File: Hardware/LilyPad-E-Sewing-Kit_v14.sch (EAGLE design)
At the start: 42 parts

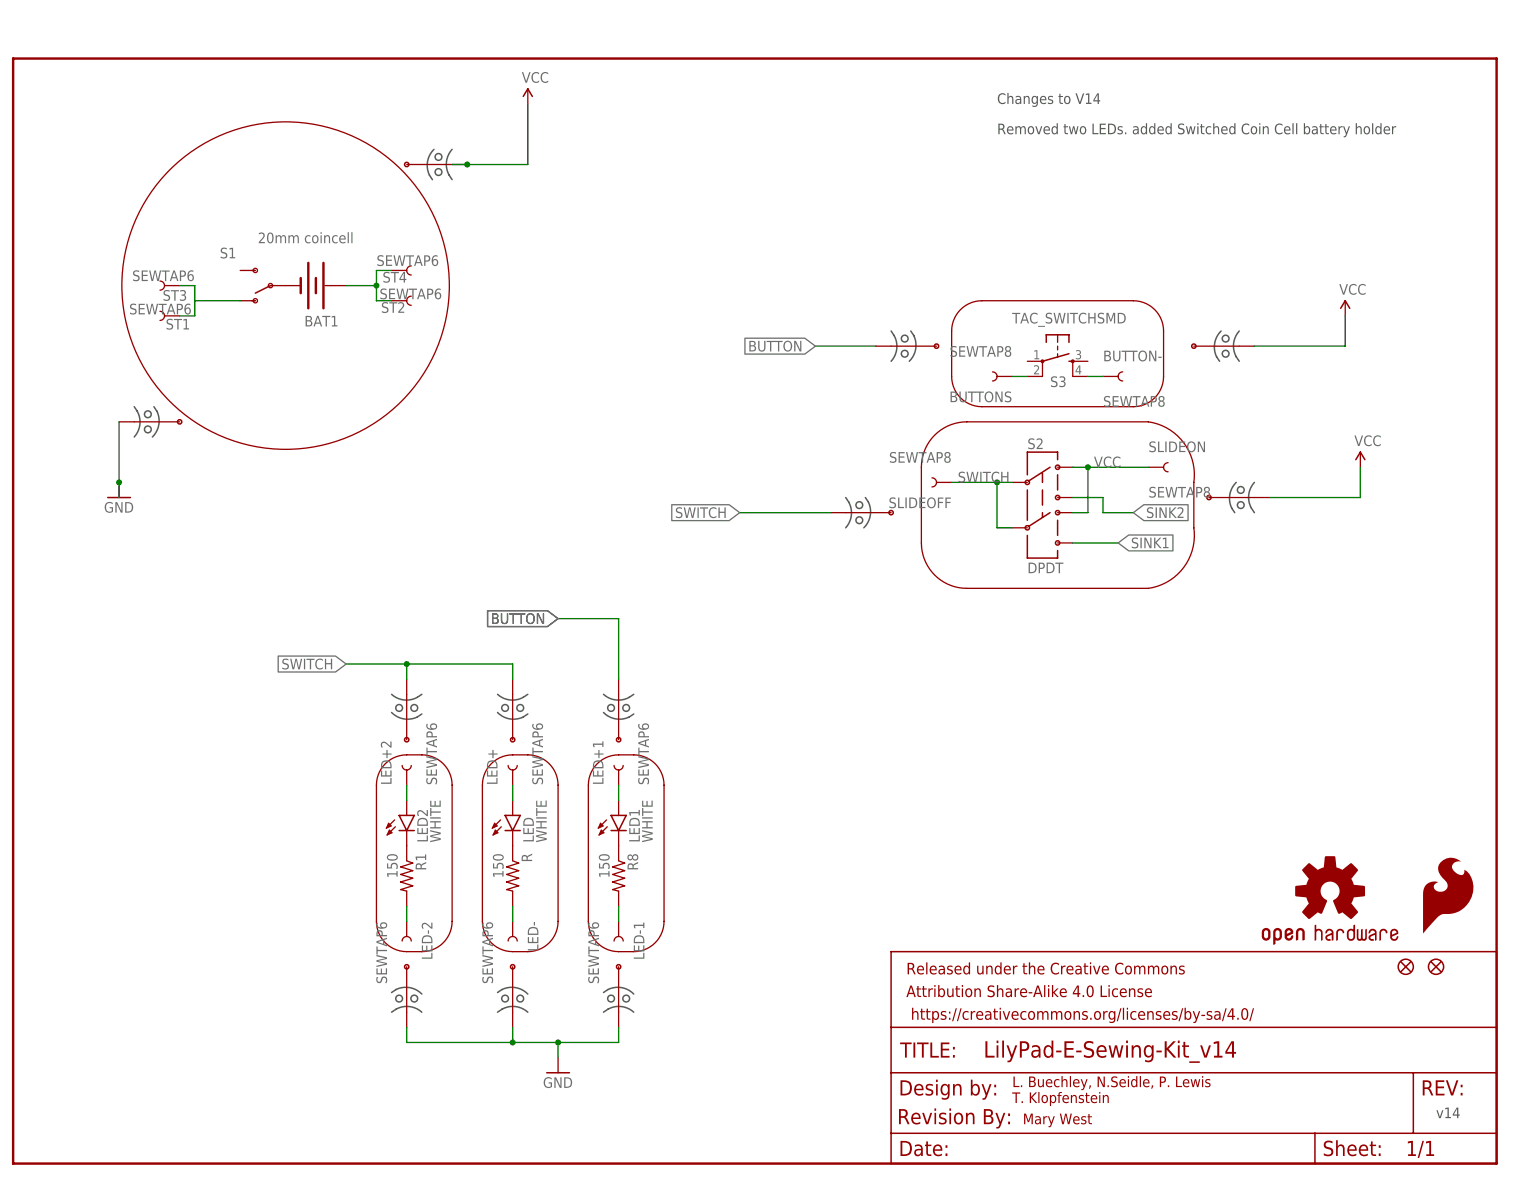
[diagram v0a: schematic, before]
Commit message: Updated Brd and Sch files (in Sync)
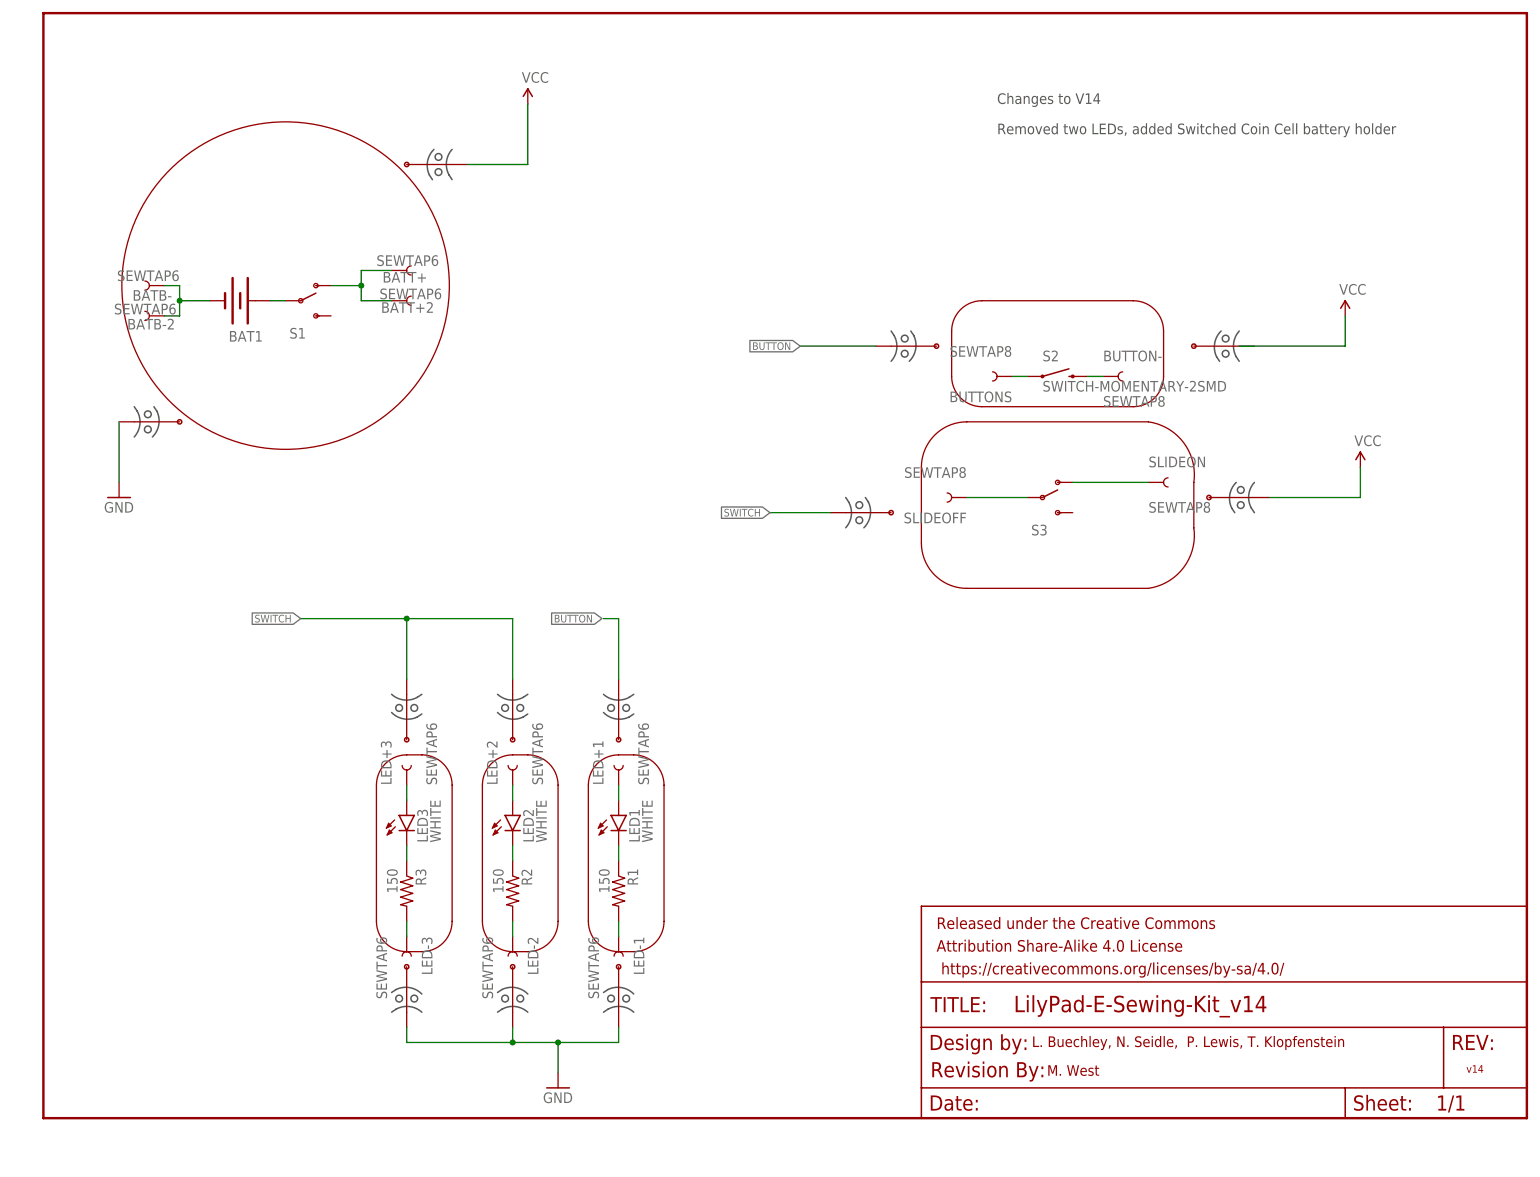
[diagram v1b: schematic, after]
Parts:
- removed JP1, JP4: FIDUCIALUFIDUCIAL, SparkFun-Aesthetics:FIDUCIALUFIDUCIAL
- removed LED: WHITE, SparkFun-LED:LED-WHITE1206
- removed LED+, LED-, ST1, ST3: SEWTAP6, LilyPad-Wearables:SEWTAP6
- removed LOGO1: SFE_LOGO_FLAME.1_STOP, SparkFun-Aesthetics:SFE_LOGO_FLAME.1_STOP
- removed R, R8: 150, SparkFun-Resistors:150OHM-1/10W-1%(0603)
- removed U$5: REVISION, SparkFun-Aesthetics:REVISION
- removed U$8: OSHW-LOGOS, SparkFun-Aesthetics:OSHW-LOGOS
- added BATB-, BATB-2, LED+3, LED-3: SEWTAP6, LilyPad-Wearables:SEWTAP6
- added LED3: WHITE, SparkFun-LED:LED-WHITE1206
- added R2, R3: 150, SparkFun-Resistors:150OHM-1/10W-1%(0603)
- added U$1: REVISION, SparkFun-Aesthetics:REVISION
- BUTTON-, BUTTONS, SLIDEOFF, SLIDEON: device LilyPad-Wearables:SEWTAP4 -> LilyPad-Wearables:SEWTAP8
- S2: value DPDT -> SWITCH-MOMENTARY-2SMD; device SparkFun-Electromechanical:SWITCH-DPDTAYZ0202 -> SparkFun-Electromechanical:SWITCH-MOMENTARY-2SMD
- S3: value TAC_SWITCHSMD -> (none); device SparkFun-Retired:TAC_SWITCHSMD -> SparkFun-Electromechanical:SWITCH-SPDTSMD
- renumbered ST2 to BATT+2, ST4 to BATT+, U$10 to MB6, U$13 to MB3, U$14 to MB4, U$18 to MB8, U$19 to MB7, U$40 to MB2, U$42 to MB9, U$44 to MB10, U$46 to MB1, U$6 to MB+, U$7 to MB-, U$9 to MB5
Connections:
- removed net GND1: LED-2.1, R1.2
- removed net N$18: LED.C, R.1
- removed net N$21: LED1.C, R8.1
- removed net SINK1: S2.6
- removed net SINK2: S2.3
- removed net SWITCH1: LED+2.1, LED2.A
- removed net VCC: BAT1.+, BATT+.1, BATT+2.1, BUTTON-.1, MB+.P$1, MB1.P$1, MB2.P$1, S2.1, S2.4, S3.4, SLIDEON.1
- new net N$11: LED1.C, R1.1
- new net N$12: LED2.C, R2.1
- new net N$13: LED3.C, R3.1
- net BUTTON: now also S2.1; no longer S3.2
- net GND: now also BAT1.-, BATB-.1, BATB-2.1, LED-2.1, LED-3.1, R1.2, R2.2, R3.2; no longer LED-.1, R.2, R8.2, S1.O, ST1.1, ST3.1
- net N$1: now also BAT1.+; no longer BAT1.-
- net N$2: now also BATT+.1, BATT+2.1, BUTTON-.1, MB+.P$1, MB1.P$1, S1.O, S2.2, S3.O, SLIDEON.1; no longer LED2.C, R1.1
- net SWITCH: now also LED+2.1, LED+3.1, LED2.A, LED3.A, S3.P; no longer LED+.1, LED.A, S2.2, S2.5
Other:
- note added: "L. Buechley, N. Seidle, P. Lewis, T. Klopfenstein"
- note added: "M. West"
- note added: "Removed two LEDs, added Switched Coin Cell battery holder"
- note removed: "L. Buechley, N.Seidle, P. Lewis T. Klopfenstein"
- note removed: "Mary West"
- note removed: "Removed two LEDs. added Switched Coin Cell battery holder"
- moved on the sheet: BAT1, LED+2, LED-1, LED-2, LED2, R1, S1, SLIDEOFF, SLIDEON
